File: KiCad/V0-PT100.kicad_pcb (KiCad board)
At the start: 2 copper layers, 21 parts, among them J1 T1, J2 T2, J3 SPI1, J4 Servos, U1 MAX31865ATP+, U2 MIC5225-3.3YM5-TR

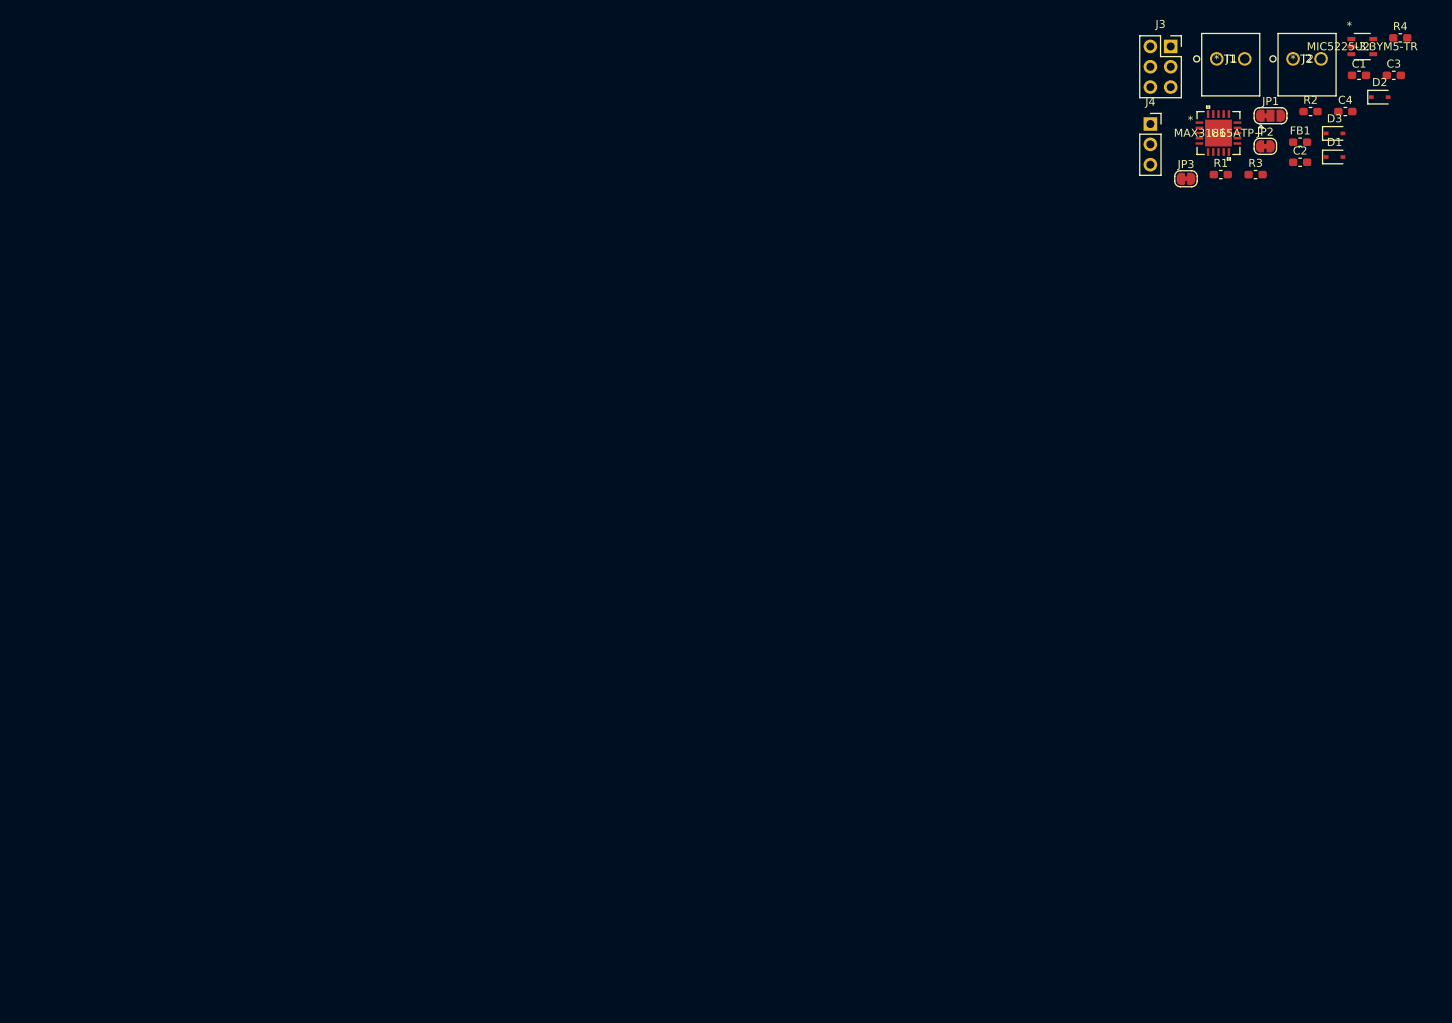
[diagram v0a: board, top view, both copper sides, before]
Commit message: Inital PCB layout complete
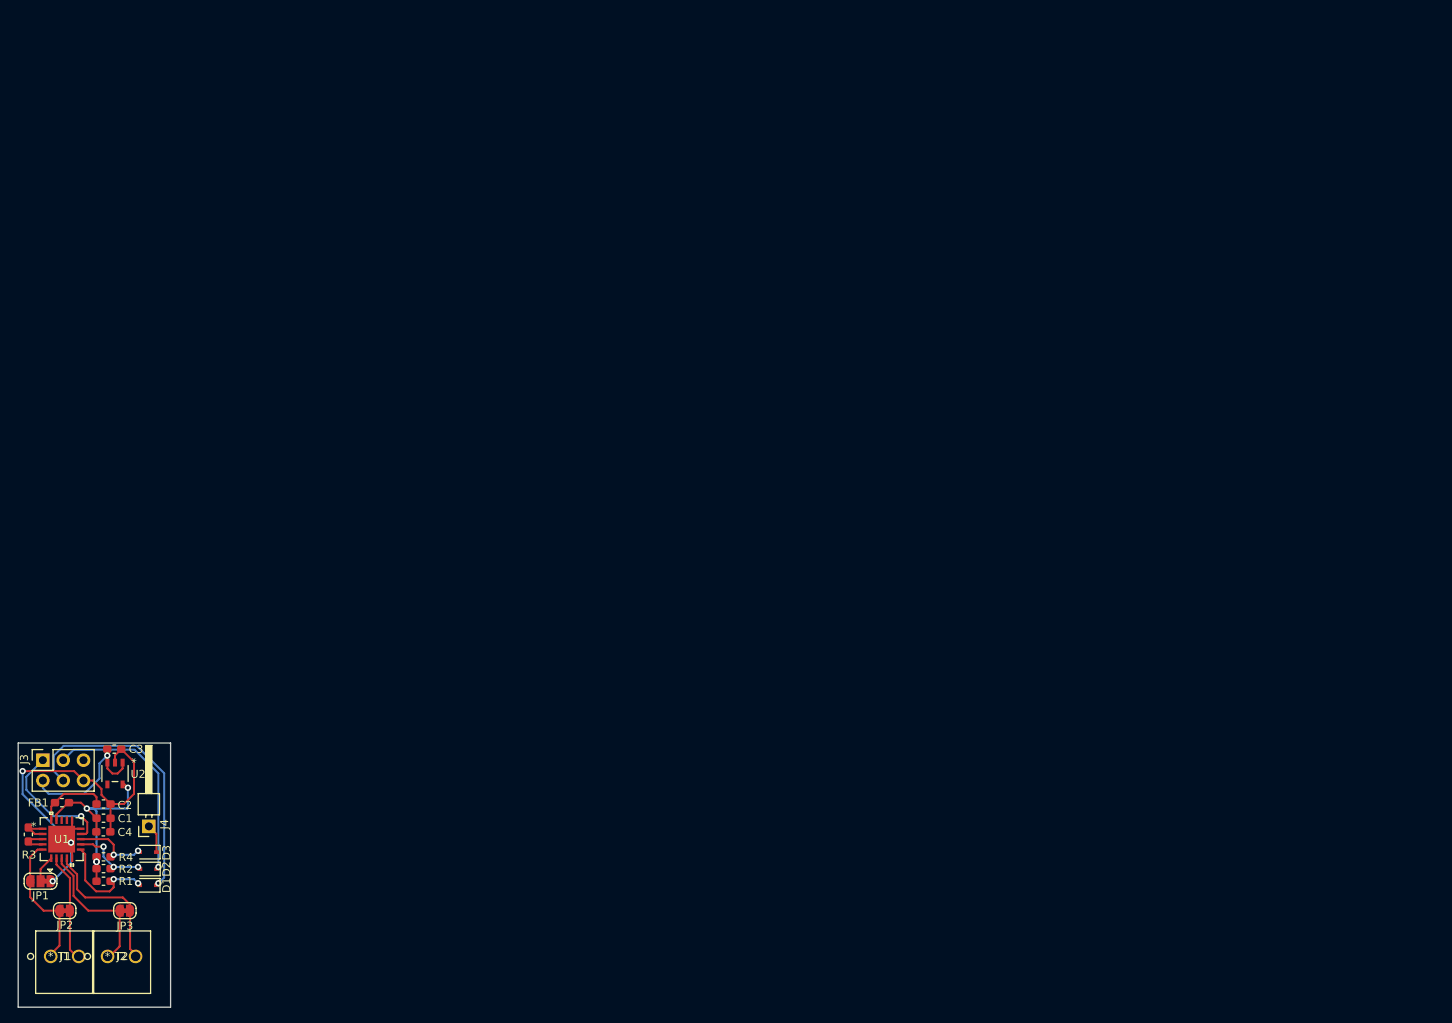
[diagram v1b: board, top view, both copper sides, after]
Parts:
- J4: value Servos -> Output; footprint Connector_PinSocket_2.54mm:PinSocket_1x03_P2.54mm_Vertical -> Connector_PinHeader_2.54mm:PinHeader_1x01_P2.54mm_Horizontal
- moved R4 191.7 mm to (114.8, 122.2), turned to 180 degrees
- moved J2 185.9 mm to (115.3, 134.6)
- moved J1 183.9 mm to (108.2, 134.6)
- moved C1 182.4 mm to (114.8, 117.3)
- moved D2 181.7 mm to (120.4, 123.7), turned to 180 degrees
- moved JP1 181.1 mm to (106.9, 125.2), turned to 180 degrees
- moved C3 180.8 mm to (116.2, 108.7)
- moved U2 180.5 mm to (116.2, 111.8), turned to 270 degrees
- moved C4 179.5 mm to (114.8, 119.0)
- moved R2 178.1 mm to (114.8, 123.6), turned to 180 degrees
- moved JP2 177.9 mm to (110.0, 128.9), turned to 180 degrees
- moved FB1 175.4 mm to (109.6, 115.4), turned to 180 degrees
- moved R3 174.2 mm to (105.4, 119.4), turned to 90 degrees
- moved D1 174.0 mm to (120.4, 125.7), turned to 180 degrees
- moved D3 173.4 mm to (120.4, 121.6), turned to 180 degrees
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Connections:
- net Net-(C2-Pad1) renamed /VDD
- net Net-(R3-Pad1) renamed /ISENSOR
- net Net-(R3-Pad2) renamed /BIAS
- J1 pad 1: /M-RTDIN+ -> /FORCE+
- J1 pad 2: /FORCE+ -> /M-RTDIN+
- J2 pad 1: /FORCE- -> /M-RTDIN-
- J2 pad 2: /M-RTDIN- -> /FORCE-
- J4 pad 1: GND -> /CS
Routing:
- net GND: track 0.00 -> 52.7 mm, vias 0 -> 3
- net /SDI: track 0.00 -> 33.4 mm, vias 0 -> 1
- net +3V3: track 0.00 -> 28.1 mm, vias 0 -> 4
- net /SCK: track 0.00 -> 25.4 mm, vias 0 -> 1
- net +5V: track 0.00 -> 19.6 mm, vias 0 -> 1
- net /FORCE-: track 0.00 -> 18.7 mm
- net /M-RTDIN-: track 0.00 -> 18.1 mm
- net /FORCE+: track 0.00 -> 17.6 mm
- net /SDO: track 0.00 -> 16.0 mm, vias 0 -> 1
- net /M-RTDIN+: track 0.00 -> 13.3 mm
- net /M-SDI: track 0.00 -> 12.7 mm, vias 0 -> 2
- net /M-SCK: track 0.00 -> 9.35 mm, vias 0 -> 3
- net /VDD: track 0.00 -> 9.07 mm
- net /M-CS: track 0.00 -> 8.94 mm, vias 0 -> 2
- net /M-FORCE2: track 0.00 -> 4.10 mm
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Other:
- board outline added: 19 x 33 mm
